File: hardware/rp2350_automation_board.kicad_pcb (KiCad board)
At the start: 2 copper layers, 6 parts, among them Q1 FCX690BTA, U1 XTR117AIDGKR, U2 ISO7041FDBQR, U3 Pico, U4 DAC60501MDGSR, U5 INA219AIDCNR

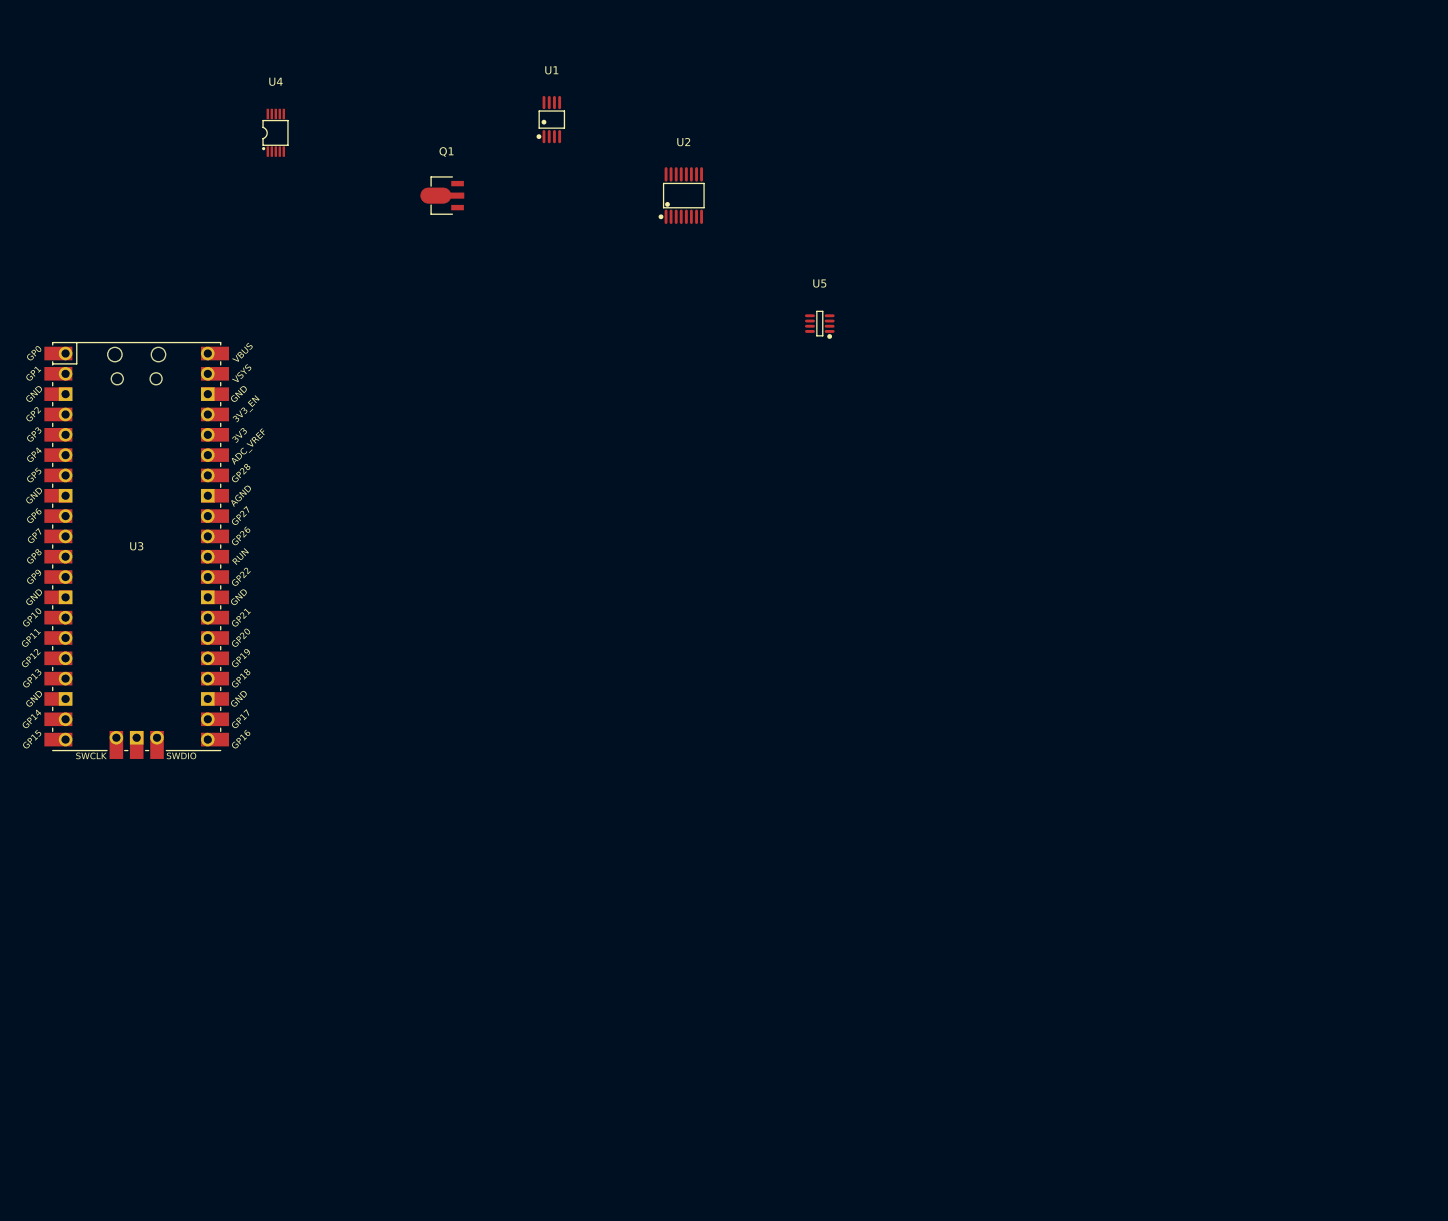
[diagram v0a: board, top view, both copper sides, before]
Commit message: Almost everything
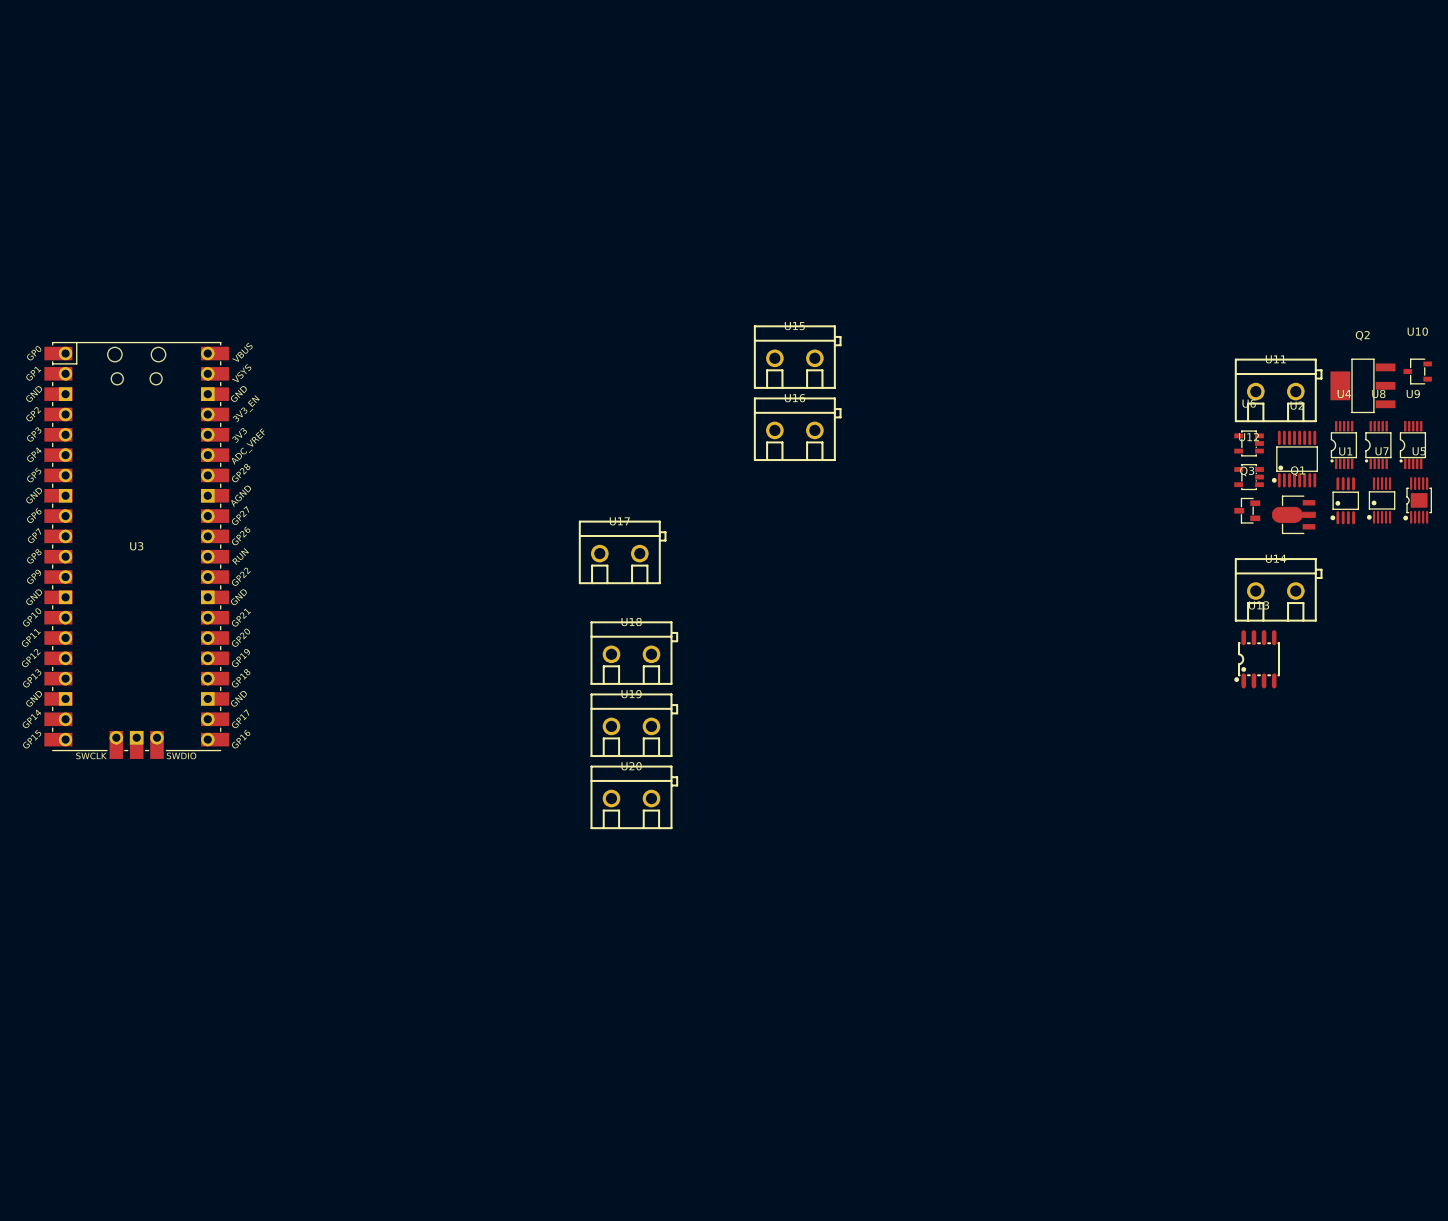
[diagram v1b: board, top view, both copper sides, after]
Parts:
- added Q2: NTF2955T1G, EasyEDA:SOT-223-4_L6.5-W3.5-P2.30-LS7.0-BR, F.Cu at (198.9, 65.3)
- added Q3: MMBT2907ALT1G, EasyEDA:SOT-23-3_L2.9-W1.3-P1.90-LS2.4-BR, F.Cu at (184.4, 80.9)
- added U10: REF3040AIDBZR, EasyEDA:SOT-23-3_L2.9-W1.6-P1.90-LS2.8-BR, F.Cu at (205.7, 63.5)
- added U11: KF301-5.0-2P, EasyEDA:CONN-TH_P5.00_KF301-5.0-2P, F.Cu at (188.0, 66.0)
- added U12: TLV9301IDBVR, EasyEDA:SOT-23-5_L3.0-W1.7-P0.95-LS2.8-BR, F.Cu at (184.7, 76.7)
- added U13: MAX3485AEASA+T, EasyEDA:SO-8_L4.9-W3.9-P1.27-LS5.9-BL, F.Cu at (185.9, 99.5)
- added U14: KF301-5.0-2P, EasyEDA:CONN-TH_P5.00_KF301-5.0-2P, F.Cu at (188.0, 90.9)
- added U15: KF301-5.0-2P, EasyEDA:CONN-TH_P5.00_KF301-5.0-2P, F.Cu at (127.9, 61.8)
- added U16: KF301-5.0-2P, EasyEDA:CONN-TH_P5.00_KF301-5.0-2P, F.Cu at (127.9, 70.9)
- added U17: KF301-5.0-2P, EasyEDA:CONN-TH_P5.00_KF301-5.0-2P, F.Cu at (106.0, 86.2)
- added U18: KF301-5.0-2P, EasyEDA:CONN-TH_P5.00_KF301-5.0-2P, F.Cu at (107.5, 98.8)
- added U19: KF301-5.0-2P, EasyEDA:CONN-TH_P5.00_KF301-5.0-2P, F.Cu at (107.5, 107.9)
- added U20: KF301-5.0-2P, EasyEDA:CONN-TH_P5.00_KF301-5.0-2P, F.Cu at (107.5, 116.9)
- added U6: TLV9301IDBVR, EasyEDA:SOT-23-5_L3.0-W1.7-P0.95-LS2.8-BR, F.Cu at (184.7, 72.5)
- added U7: INA226AIDGSR, EasyEDA:MSOP-10_L3.0-W3.0-P0.50-LS5.0-BL, F.Cu at (201.3, 79.6)
- added U8: DAC60501MDGSR, EasyEDA:VSSOP-10_L3.0-W3.0-P0.50-LS4.9-BL, F.Cu at (200.9, 72.7)
- added U9: DAC60501MDGSR, EasyEDA:VSSOP-10_L3.0-W3.0-P0.50-LS4.9-BL, F.Cu at (205.2, 72.7)
- U5: value INA219AIDCNR -> XTR111AIDGQR; footprint EasyEDA:SOT-23-8_L3.0-W1.7-P0.65-LS2.8-BR -> EasyEDA:MSOP-10_L3.0-W3.0-P0.50-LS5.0-BL-EP
- moved U4 139.1 mm to (196.6, 72.7)
- moved Q1 113.7 mm to (190.8, 81.4)
- moved U1 110.1 mm to (196.7, 79.6)
- moved U2 83.4 mm to (190.7, 74.4)
- moved U5 78.1 mm to (205.9, 79.6)
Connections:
- U1 pad 2: unconnected-(U1-IIN-Pad2) -> Net-(U1-IIN)
- U2 pad 1: unconnected-(U2-VCC1-Pad1) -> +5V_MCU
- U2 pad 10: unconnected-(U2-EN2-Pad10) -> GND_XTR
- U2 pad 12: unconnected-(U2-OUTC-Pad12) -> Net-(U2-OUTC)
- U2 pad 13: unconnected-(U2-OUTB-Pad13) -> Net-(U2-OUTB)
- U2 pad 14: unconnected-(U2-OUTA-Pad14) -> Net-(U2-OUTA)
- U2 pad 16: unconnected-(U2-VCC2-Pad16) -> 5V_XTR
- U2 pad 3: unconnected-(U2-INA-Pad3) -> SPI0_CLK
- U2 pad 4: unconnected-(U2-INB-Pad4) -> SPI0_CS
- U2 pad 5: unconnected-(U2-INC-Pad5) -> SPI0_MOSI
- U2 pad 6: unconnected-(U2-OUTD-Pad6) -> SPI0_MISO
- U2 pad 7: unconnected-(U2-EN1-Pad7) -> GND_MCU
- U2 pad 8: unconnected-(U2-GND1-Pad8) -> GND_MCU
- U2 pad 9: unconnected-(U2-GND2-Pad9) -> GND_XTR
- U3 pad 21: SPI0_MISO -> UART_TX
- U3 pad 22: SPI0_CS -> UART_RX
- U3 pad 24: SPI0_CLK -> RS485_MODE
- U3 pad 25: SPI0_MOSI -> unconnected-(U3-GPIO19-Pad25)
- U3 pad 26: unconnected-(U3-GPIO20-Pad26) -> SDA
- U3 pad 27: unconnected-(U3-GPIO21-Pad27) -> SCL
- U3 pad 31: unconnected-(U3-GPIO26_ADC0-Pad31) -> ADC0
- U3 pad 36: +3V3_MCU -> +3V3
- U3 pad 39: unconnected-(U3-VSYS-Pad39) -> VSYS
- U3 pad 40: +5V_MCU -> unconnected-(U3-VBUS-Pad40)_1
- U4 pad 1: unconnected-(U4-VDD-Pad1) -> 5V_XTR
- U4 pad 2: unconnected-(U4-VOUT-Pad2) -> Net-(U4-VOUT)
- U4 pad 4: unconnected-(U4-AGND-Pad4) -> GND_XTR
- U4 pad 5: unconnected-(U4-SPI2C-Pad5) -> Net-(U4-SPI2C)
- U4 pad 6: unconnected-(U4-SCLK/SCL-Pad6) -> Net-(U2-OUTA)
- U4 pad 7: unconnected-(U4-~{SYNC}/A0-Pad7) -> Net-(U2-OUTB)
- U4 pad 8: unconnected-(U4-SDIN/SDA-Pad8) -> Net-(U2-OUTC)
- U5 pad 1: unconnected-(U5-IN+-Pad1) -> +12V
- U5 pad 2: unconnected-(U5-IN--Pad2) -> Net-(Q3-E)
- U5 pad 3: unconnected-(U5-GND-Pad3) -> Net-(Q3-C)
- U5 pad 4: unconnected-(U5-VS-Pad4) -> Net-(U5-REGS)
- U5 pad 5: unconnected-(U5-SCL-Pad5) -> Net-(U5-REGF)
- U5 pad 6: unconnected-(U5-SDA-Pad6) -> Net-(U5-VIN)
- U5 pad 7: unconnected-(U5-A0-Pad7) -> Net-(U5-SET)

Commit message: Board complete
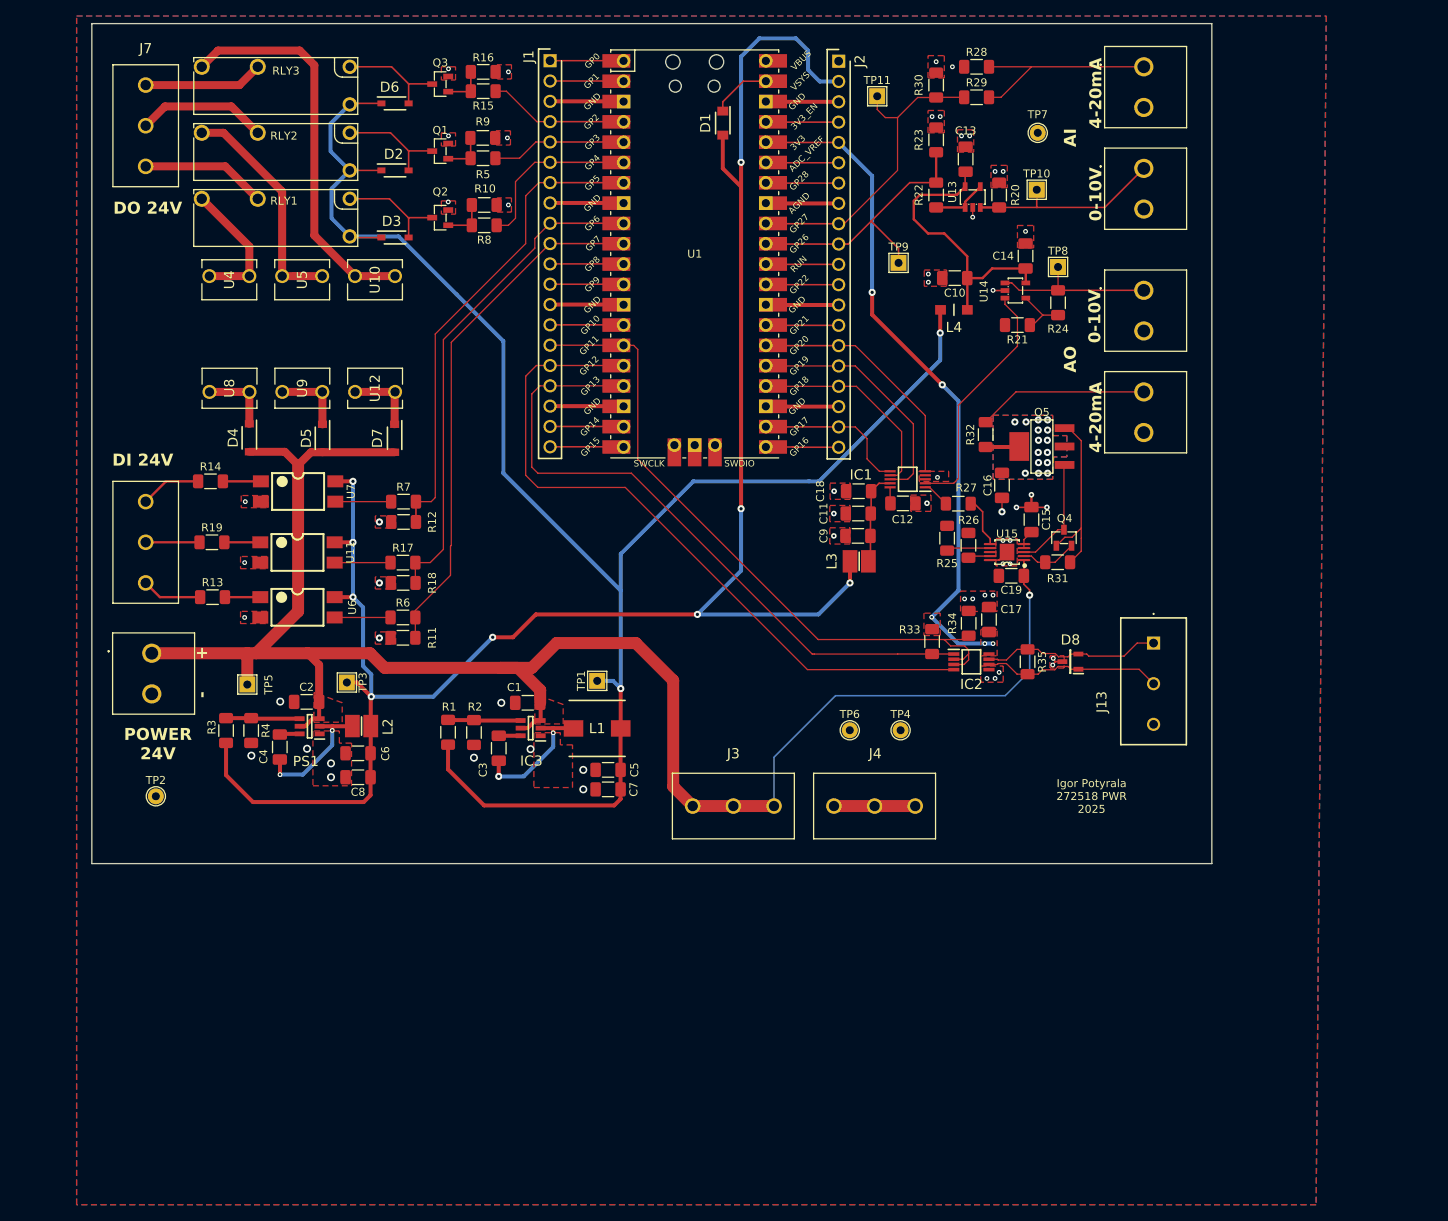
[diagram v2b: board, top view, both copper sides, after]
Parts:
- removed U16, U17, U18, U19, U20: KF301-5.0-2P, EasyEDA:CONN-TH_P5.00_KF301-5.0-2P
- removed U2: ISO7041FDBQR, EasyEDA:SSOP-16_L4.9-W3.9-P0.64-LS6.0-BL
- removed U3: Pico, MCU_RaspberryPi_and_Boards:RPi_Pico_SMD_TH
- added C1: 2.2uF, Capacitor_SMD:C_1206_3216Metric_Pad1.33x1.80mm_HandSolder, F.Cu at (94.5, 104.9)
- added C10: 10uF, Capacitor_SMD:C_1206_3216Metric_Pad1.33x1.80mm_HandSolder, F.Cu at (147.9, 51.8)
- added C11: 1uF, Capacitor_SMD:C_1206_3216Metric_Pad1.33x1.80mm_HandSolder, F.Cu at (135.8, 81.2)
- added C12: 150nF, Capacitor_SMD:C_1206_3216Metric_Pad1.33x1.80mm_HandSolder, F.Cu at (141.4, 80.0)
- added C13: 0.1uF, Capacitor_SMD:C_1206_3216Metric_Pad1.33x1.80mm_HandSolder, F.Cu at (149.2, 36.9)
- added C14: 0.1uF, Capacitor_SMD:C_1206_3216Metric_Pad1.33x1.80mm_HandSolder, F.Cu at (156.7, 49.0)
- added C15: 470nF, Capacitor_SMD:C_1206_3216Metric_Pad1.33x1.80mm_HandSolder, F.Cu at (157.5, 82.0)
- added C16: 10nF, Capacitor_SMD:C_1206_3216Metric_Pad1.33x1.80mm_HandSolder, F.Cu at (153.8, 77.7)
- added C17: C, Capacitor_SMD:C_1206_3216Metric_Pad1.33x1.80mm_HandSolder, F.Cu at (152.1, 94.5)
- added C18: 1nF, Capacitor_SMD:C_1206_3216Metric_Pad1.33x1.80mm_HandSolder, F.Cu at (135.9, 78.5)
- added C19: 0.1uF, Capacitor_SMD:C_1206_3216Metric_Pad1.33x1.80mm_HandSolder, F.Cu at (154.9, 89.0)
- added C2: 2.2uF, Capacitor_SMD:C_1206_3216Metric_Pad1.33x1.80mm_HandSolder, F.Cu at (66.9, 104.8)
- added C3: 0.1uF, Capacitor_SMD:C_1206_3216Metric_Pad1.33x1.80mm_HandSolder, F.Cu at (90.9, 110.6)
- added C4: 0.1uF, Capacitor_SMD:C_1206_3216Metric_Pad1.33x1.80mm_HandSolder, F.Cu at (63.5, 110.4)
- added C5: 22uF, Capacitor_SMD:C_1206_3216Metric_Pad1.33x1.80mm_HandSolder, F.Cu at (104.5, 113.3)
- added C6: 10uF, Capacitor_SMD:C_1206_3216Metric_Pad1.33x1.80mm_HandSolder, F.Cu at (73.3, 111.2)
- added C7: 22uF, Capacitor_SMD:C_1206_3216Metric_Pad1.33x1.80mm_HandSolder, F.Cu at (104.5, 115.7)
- added C8: 10uF, Capacitor_SMD:C_1206_3216Metric_Pad1.33x1.80mm_HandSolder, F.Cu at (73.3, 114.2)
- added C9: 10uF, Capacitor_SMD:C_1206_3216Metric_Pad1.33x1.80mm_HandSolder, F.Cu at (135.8, 84.0)
- added D1: MBR230S1F-7, Samacsys:SODFL3518X115N, F.Cu at (118.9, 32.4)
- added D2: 1N4148W, Samacsys:SODFL3816X120N, F.Cu at (77.9, 38.4)
- added D3: 1N4148W, Samacsys:SODFL3816X120N, F.Cu at (77.9, 46.7)
- added D4: 1N4007W-T, Samacsys:SODFL3818X130N, F.Cu at (59.7, 71.8)
- added D5: 1N4007W-T, Samacsys:SODFL3818X130N, F.Cu at (68.8, 71.8)
- added D6: 1N4148W, Samacsys:SODFL3816X120N, F.Cu at (77.9, 30.0)
- added D7: 1N4007W-T, Samacsys:SODFL3818X130N, F.Cu at (77.9, 71.8)
- added D8: CDSOT23-SM712, Samacsys:SOT95P230X117-3N, F.Cu at (162.3, 99.8)
- added IC1: DAC7562SDGSR, Samacsys:SOP50P490X110-10N, F.Cu at (142.0, 77.0)
- added IC2: SN65HVD75DGKR, Samacsys:SOP65P490X110-8N, F.Cu at (149.9, 99.8)
- added IC3: LMR51420XFDDCR, Samacsys:SOT95P280X110-6N, F.Cu at (94.9, 108.1)
- added J1: PH1-20-UA, Samacsys:HDRV20W64P0X254_1X20_5080X249X886P, F.Cu at (97.3, 24.6)
- added J10: TB007-508-02BE, Samacsys:TB00750802BE, F.Cu at (171.5, 53.3)
- added J11: TB007-508-02BE, Samacsys:TB00750802BE, F.Cu at (171.5, 25.4)
- added J12: TB007-508-02BE, Samacsys:TB00750802BE, F.Cu at (171.5, 66.0)
- added J13: 39880-0303, Samacsys:398800303, F.Cu at (172.7, 97.4)
- added J14: TB006-508-03BE, Samacsys:TB00650803BE, F.Cu at (46.7, 89.9)
- added J2: PH1-20-UA, Samacsys:HDRV20W64P0X254_1X20_5080X249X886P, F.Cu at (133.4, 24.7)
- added J3: TB006-508-03BE, Samacsys:TB00650803BE, F.Cu at (125.3, 117.8)
- added J4: TB006-508-03BE, Samacsys:TB00650803BE, F.Cu at (132.8, 117.8)
- added J5: TB007-508-02BE, Samacsys:TB00750802BE, F.Cu at (47.5, 98.7)
- added J7: TB006-508-03BE, Samacsys:TB00650803BE, F.Cu at (46.7, 37.8)
- added J9: TB007-508-02BE, Samacsys:TB00750802BE, F.Cu at (171.5, 38.1)
- added L1: 22uH, Samacsys:INDPM7070X480N, F.Cu at (103.2, 108.1)
- added L2: 4.7uH, Samacsys:INDC3225X120N, F.Cu at (73.7, 107.8)
- added L3: 4.7uH, Samacsys:INDC3225X120N, F.Cu at (135.9, 87.2)
- added L4: 1uH, Samacsys:LQM31PN1R0M00L, F.Cu at (147.8, 55.8)
- added PS1: LMR51420YFDDCR, Samacsys:SOT95P280X110-6N, F.Cu at (67.2, 107.8)
- added Q4: MMBT2907ALT1G, EasyEDA:SOT-23-3_L2.9-W1.3-P1.90-LS2.4-BR, F.Cu at (161.5, 84.3)
- added Q5: BSP171PH6327XTSA1, EasyEDA:SOT-223-4_L6.5-W3.5-P2.30-LS7.0-BR, F.Cu at (158.8, 72.9)
- added R1: 100k, Resistor_SMD:R_1206_3216Metric_Pad1.30x1.75mm_HandSolder, F.Cu at (84.5, 108.6)
- added R10: 10k, Resistor_SMD:R_1206_3216Metric_Pad1.30x1.75mm_HandSolder, F.Cu at (89.1, 42.7)
- added R11: 20k, Resistor_SMD:R_1206_3216Metric_Pad1.30x1.75mm_HandSolder, F.Cu at (78.9, 96.8)
- added R12: 20k, Resistor_SMD:R_1206_3216Metric_Pad1.30x1.75mm_HandSolder, F.Cu at (79.0, 82.3)
- added R13: 3.3k, Resistor_SMD:R_1206_3216Metric_Pad1.30x1.75mm_HandSolder, F.Cu at (55.1, 91.7)
- added R14: 3.3k, Resistor_SMD:R_1206_3216Metric_Pad1.30x1.75mm_HandSolder, F.Cu at (54.8, 77.2)
- added R15: 330, Resistor_SMD:R_1206_3216Metric_Pad1.30x1.75mm_HandSolder, F.Cu at (88.9, 28.4)
- added R16: 10k, Resistor_SMD:R_1206_3216Metric_Pad1.30x1.75mm_HandSolder, F.Cu at (88.9, 26.0)
- added R17: 10k, Resistor_SMD:R_1206_3216Metric_Pad1.30x1.75mm_HandSolder, F.Cu at (78.9, 87.4)
- added R18: 20k, Resistor_SMD:R_1206_3216Metric_Pad1.30x1.75mm_HandSolder, F.Cu at (78.9, 89.9)
- added R19: 3.3k, Resistor_SMD:R_1206_3216Metric_Pad1.30x1.75mm_HandSolder, F.Cu at (55.0, 84.8)
- added R2: 5.23k, Resistor_SMD:R_1206_3216Metric_Pad1.30x1.75mm_HandSolder, F.Cu at (87.8, 108.6)
- added R20: 100k, Resistor_SMD:R_1206_3216Metric_Pad1.30x1.75mm_HandSolder, F.Cu at (153.4, 41.4)
- added R21: 10k, Resistor_SMD:R_1206_3216Metric_Pad1.30x1.75mm_HandSolder, F.Cu at (155.7, 57.7)
- added R22: 56k, Resistor_SMD:R_1206_3216Metric_Pad1.30x1.75mm_HandSolder, F.Cu at (145.5, 41.4)
- added R23: 24k, Resistor_SMD:R_1206_3216Metric_Pad1.30x1.75mm_HandSolder, F.Cu at (145.5, 34.5)
- added R24: 30k, Resistor_SMD:R_1206_3216Metric_Pad1.30x1.75mm_HandSolder, F.Cu at (160.8, 54.9)
- added R25: 1.25k, Resistor_SMD:R_1206_3216Metric_Pad1.30x1.75mm_HandSolder, F.Cu at (146.9, 84.3)
- added R26: 10k, Resistor_SMD:R_1206_3216Metric_Pad1.30x1.75mm_HandSolder, F.Cu at (149.6, 85.2)
- added R27: 0R, Resistor_SMD:R_1206_3216Metric_Pad1.30x1.75mm_HandSolder, F.Cu at (148.3, 80.0)
- added R28: 250R, Resistor_SMD:R_1206_3216Metric_Pad1.30x1.75mm_HandSolder, F.Cu at (150.6, 25.4)
- added R29: 22k, Resistor_SMD:R_1206_3216Metric_Pad1.30x1.75mm_HandSolder, F.Cu at (150.6, 29.2)
- added R3: 100k, Resistor_SMD:R_1206_3216Metric_Pad1.30x1.75mm_HandSolder, F.Cu at (56.8, 108.4)
- added R30: 33k, Resistor_SMD:R_1206_3216Metric_Pad1.30x1.75mm_HandSolder, F.Cu at (145.5, 27.7)
- added R31: 15, Resistor_SMD:R_1206_3216Metric_Pad1.30x1.75mm_HandSolder, F.Cu at (160.7, 87.3)
- added R32: 15, Resistor_SMD:R_1206_3216Metric_Pad1.30x1.75mm_HandSolder, F.Cu at (151.7, 71.4)
- added R33: 10k, Resistor_SMD:R_1206_3216Metric_Pad1.30x1.75mm_HandSolder, F.Cu at (145.0, 97.2)
- added R34: 10k, Resistor_SMD:R_1206_3216Metric_Pad1.30x1.75mm_HandSolder, F.Cu at (149.6, 95.0)
- added R35: 120R, Resistor_SMD:R_1206_3216Metric_Pad1.30x1.75mm_HandSolder, F.Cu at (157.0, 99.8)
- added R4: 13.7k, Resistor_SMD:R_1206_3216Metric_Pad1.30x1.75mm_HandSolder, F.Cu at (59.9, 108.4)
- added R5: 330, Resistor_SMD:R_1206_3216Metric_Pad1.30x1.75mm_HandSolder, F.Cu at (88.9, 36.8)
- added R6: 10k, Resistor_SMD:R_1206_3216Metric_Pad1.30x1.75mm_HandSolder, F.Cu at (78.9, 94.2)
- added R7: 10k, Resistor_SMD:R_1206_3216Metric_Pad1.30x1.75mm_HandSolder, F.Cu at (79.0, 79.8)
- added R8: 330, Resistor_SMD:R_1206_3216Metric_Pad1.30x1.75mm_HandSolder, F.Cu at (89.1, 45.2)
- added R9: 10k, Resistor_SMD:R_1206_3216Metric_Pad1.30x1.75mm_HandSolder, F.Cu at (88.9, 34.3)
- added RLY1: G5NB-1A-E-DC12, EasyEDA:RELAY-TH_G5NB-1A-E-DCXX, F.Cu at (63.0, 44.2)
- added RLY2: G5NB-1A-E-DC12, EasyEDA:RELAY-TH_G5NB-1A-E-DCXX, F.Cu at (63.0, 36.0)
- added RLY3: G5NB-1A-E-DC12, EasyEDA:RELAY-TH_G5NB-1A-E-DCXX, F.Cu at (63.0, 27.8)
- added TP1: TP_+12V, TestPoint:TestPoint_THTPad_2.0x2.0mm_Drill1.0mm, F.Cu at (103.2, 102.2)
- added TP10: TP_AI_0-10V, TestPoint:TestPoint_THTPad_2.0x2.0mm_Drill1.0mm, F.Cu at (158.1, 40.8)
- added TP11: TP_ADC1, TestPoint:TestPoint_THTPad_2.0x2.0mm_Drill1.0mm, F.Cu at (138.2, 29.1)
- added TP2: GND_TP, TestPoint:TestPoint_THTPad_D2.0mm_Drill1.0mm, F.Cu at (48.0, 116.6)
- added TP3: TP_+5V, TestPoint:TestPoint_THTPad_2.0x2.0mm_Drill1.0mm, F.Cu at (71.9, 102.4)
- added TP4: GND_TP, TestPoint:TestPoint_THTPad_D2.0mm_Drill1.0mm, F.Cu at (141.1, 108.3)
- added TP5: TP_+24V, TestPoint:TestPoint_THTPad_2.0x2.0mm_Drill1.0mm, F.Cu at (59.4, 102.6)
- added TP6: GND_TP, TestPoint:TestPoint_THTPad_D2.0mm_Drill1.0mm, F.Cu at (134.7, 108.3)
- added TP7: GND_TP, TestPoint:TestPoint_THTPad_D2.0mm_Drill1.0mm, F.Cu at (158.2, 33.7)
- added TP8: TP_AO_0-10V, TestPoint:TestPoint_THTPad_2.0x2.0mm_Drill1.0mm, F.Cu at (160.8, 50.4)
- added TP9: TP_ADC0, TestPoint:TestPoint_THTPad_2.0x2.0mm_Drill1.0mm, F.Cu at (140.8, 49.9)
- Q1: value FCX690BTA -> 2N7002; footprint EasyEDA:SOT-89-3_L4.5-W2.5-P1.50-LS4.2-BR -> EasyEDA:SOT-23-3_L2.9-W1.3-P1.90-LS2.4-BR
- Q2: value NTF2955T1G -> 2N7002; footprint EasyEDA:SOT-223-4_L6.5-W3.5-P2.30-LS7.0-BR -> EasyEDA:SOT-23-3_L2.9-W1.3-P1.90-LS2.4-BR
- Q3: value MMBT2907ALT1G -> 2N7002
- U1: value XTR117AIDGKR -> Pico; footprint EasyEDA:VSSOP-8_L3.0-W3.0-P0.65-LS5.0-BL -> RP-Pico Libraries:RPi_Pico_SMD_TH
- U10: value REF3040AIDBZR -> FUSE_C; footprint EasyEDA:SOT-23-3_L2.9-W1.6-P1.90-LS2.8-BR -> Samacsys:01110501Z
- U11: value KF301-5.0-2P -> LTV-814S-TA1; footprint EasyEDA:CONN-TH_P5.00_KF301-5.0-2P -> EasyEDA:SMD-4_L4.6-W6.5-P2.54-LS10.2-BL
- U12: value TLV9301IDBVR -> FUSE_C; footprint EasyEDA:SOT-23-5_L3.0-W1.7-P0.95-LS2.8-BR -> Samacsys:01110501Z
- U13: value MAX3485AEASA+T -> TLV9301IDBVR; footprint EasyEDA:SO-8_L4.9-W3.9-P1.27-LS5.9-BL -> EasyEDA:SOT-23-5_L3.0-W1.7-P0.95-LS2.8-BR
- U14: value KF301-5.0-2P -> TLV9301IDBVR; footprint EasyEDA:CONN-TH_P5.00_KF301-5.0-2P -> EasyEDA:SOT-23-5_L3.0-W1.7-P0.95-LS2.8-BR
- U15: value KF301-5.0-2P -> XTR111AIDGQR; footprint EasyEDA:CONN-TH_P5.00_KF301-5.0-2P -> EasyEDA:MSOP-10_L3.0-W3.0-P0.50-LS5.0-BL-EP
- U4, U8, U9: value DAC60501MDGSR -> FUSE_C; footprint EasyEDA:VSSOP-10_L3.0-W3.0-P0.50-LS4.9-BL -> Samacsys:01110501Z
- U5: value XTR111AIDGQR -> FUSE_C; footprint EasyEDA:MSOP-10_L3.0-W3.0-P0.50-LS5.0-BL-EP -> Samacsys:01110501Z
- U6: value TLV9301IDBVR -> LTV-814S-TA1; footprint EasyEDA:SOT-23-5_L3.0-W1.7-P0.95-LS2.8-BR -> EasyEDA:SMD-4_L4.6-W6.5-P2.54-LS10.2-BL
- U7: value INA226AIDGSR -> LTV-814S-TA1; footprint EasyEDA:MSOP-10_L3.0-W3.0-P0.50-LS5.0-BL -> EasyEDA:SMD-4_L4.6-W6.5-P2.54-LS10.2-BL
- moved U8 146.3 mm to (54.7, 66.0), turned to 90 degrees
- moved U9 141.5 mm to (63.8, 66.0), turned to 90 degrees
- moved U5 140.0 mm to (68.8, 51.6), turned to -90 degrees
- moved U4 138.5 mm to (59.7, 51.6), turned to -90 degrees
- moved U7 135.5 mm to (65.8, 78.5), turned to -90 degrees
- moved U10 128.4 mm to (77.9, 51.6), turned to -90 degrees
- moved U11 123.9 mm to (65.7, 86.1), turned to -90 degrees
- moved U6 120.7 mm to (65.7, 93.0), turned to -90 degrees
- moved Q2 117.2 mm to (83.5, 44.3)
- moved Q1 116.5 mm to (83.5, 35.9)
- moved Q3 114.1 mm to (83.5, 27.6)
- moved U12 112.3 mm to (72.9, 66.0), turned to 90 degrees
- moved U1 87.0 mm to (115.4, 48.8)
- moved U13 68.0 mm to (150.1, 41.7), turned to -90 degrees
- moved U14 49.7 mm to (155.4, 53.4), turned to 180 degrees
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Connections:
- Q1 pad 1: Net-(Q1-B) -> Net-(Q1-G)
- Q1 pad 2: AO_4-20mA_IN -> GND
- Q1 pad 3: Net-(Q1-E) -> Net-(D2-A)
- Q2 pad 2: unconnected-(Q2-D-Pad2) -> GND
- Q3 pad 1: Net-(Q2-G) -> Net-(Q3-G)
- Q3 pad 2: Net-(Q3-E) -> GND
- Q3 pad 3: Net-(Q3-C) -> Net-(D6-A)
- U1 pad 1: unconnected-(U1-NC-Pad1) -> Net-(U1-GPIO0)
- U1 pad 3: GND_XTR -> GND
- U1 pad 4: AO_4-20mA_OUT -> DOUT_1
- U1 pad 5: Net-(Q1-E) -> DOUT_2
- U1 pad 6: Net-(Q1-B) -> DOUT_3
- U1 pad 7: AO_4-20mA_IN -> DIN_1
- U1 pad 8: 5V_XTR -> GND
- U10 pad 1: +12V -> Net-(RLY3-Pad3)
- U10 pad 2: Net-(U10-OUT) -> Net-(RLY3-Pad3)
- U11 pad 1: unconnected-(U11-Pad1) -> Net-(R19-Pad2)
- U11 pad 2: unconnected-(U11-Pad2) -> GND
- U12 pad 1: Net-(U12--IN) -> Net-(D7-K)
- U12 pad 2: AI_4-20mA_GND -> Net-(D7-K)
- U13 pad 1: UART_RX -> Net-(U13--IN)
- U13 pad 2: RS485_MODE -> GND
- U13 pad 3: RS485_MODE -> /Analog IO/AI_0-10V_IN
- U13 pad 4: UART_TX -> Net-(U13--IN)
- U13 pad 5: AI_4-20mA_GND -> +12V_LPF_OP
- U14 pad 1: RS485_B -> /Analog IO/AO_0-10V
- U14 pad 2: RS485_A -> GND
- U15 pad 1: +12V -> +24V
- U15 pad 2: +12V -> Net-(Q4-E)
- U4 pad 1: 5V_XTR -> Net-(RLY1-Pad3)
- U4 pad 2: Net-(U4-VOUT) -> Net-(RLY1-Pad3)
- U5 pad 1: +12V -> Net-(RLY2-Pad3)
- U5 pad 2: Net-(Q3-E) -> Net-(RLY2-Pad3)
- U6 pad 1: AO_0-10V_OUT -> Net-(R13-Pad2)
- U6 pad 2: AI_4-20mA_GND -> GND
- U6 pad 3: Net-(U6-+IN) -> Net-(R6-Pad1)
- U6 pad 4: Net-(U6--IN) -> +5V
- U7 pad 1: AI_4-20mA_GND -> Net-(R14-Pad2)
- U7 pad 2: AI_4-20mA_GND -> GND
- U7 pad 3: unconnected-(U7-Alert-Pad3) -> Net-(R7-Pad1)
- U7 pad 4: SDA -> +5V
- U8 pad 1: +12V -> Net-(D4-K)
- U8 pad 2: Net-(U6-+IN) -> Net-(D4-K)
- U9 pad 1: +12V -> Net-(D5-K)
- U9 pad 2: Net-(U9-VOUT) -> Net-(D5-K)
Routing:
- net +5V: track 0.00 -> 239.2 mm, vias 0 -> 9
- net +24V: track 0.00 -> 226.6 mm, vias 0 -> 1
- net +12V: track 0.00 -> 211.4 mm, vias 0 -> 2
- net GND: track 0.00 -> 98.8 mm, vias 0 -> 57
- net UART_TX: track 0.00 -> 88.8 mm
- net +3V3: track 0.00 -> 85.2 mm, vias 0 -> 5
- net RS485_MODE: track 0.00 -> 84.9 mm
- net UART_RX: track 0.00 -> 83.5 mm
- net DIN_3: track 0.00 -> 65.5 mm
- net DIN_2: track 0.00 -> 62.2 mm
- net DIN_1: track 0.00 -> 61.2 mm
- net Net-(RLY3-Pad3): track 0.00 -> 49.1 mm
- net ADC1: track 0.00 -> 39.6 mm
- net +12V_LPF_OP: track 0.00 -> 36.3 mm
- net ADC0: track 0.00 -> 35.4 mm
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- added copper zone on F.Cu, net +24V
- added copper zone on F.Cu, net +3V3
- added copper zone on B.Cu, net GND
- added copper zone on F.Cu, net GND
- added copper zone on B.Cu, net Net-(C16-Pad2)
- added copper zone on F.Cu, net Net-(C16-Pad2)
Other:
- board outline added: 140 x 105 mm
- board text added: "+"
- board text added: "-"
- board text added: "0-10V"
- board text added: "4-20mA"
- board text added: "AI"
- board text added: "AO"
- board text added: "DI 24V"
- board text added: "DO 24V"
- board text added: "Igor Potyrala 272518 PWR 2025"
- board text added: "POWER 24V"
